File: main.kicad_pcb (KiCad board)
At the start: 2 copper layers, 120 x 100 mm, 21 parts, among them J1 Conn_01x01_Female, J2 Conn_01x01_Female, J3 Conn_01x01_Female, J4 Conn_01x01_Female, J5 Conn_01x01_Female, J6 Conn_01x01_Female, J7 Conn_Coaxial, Q1 AOT2618

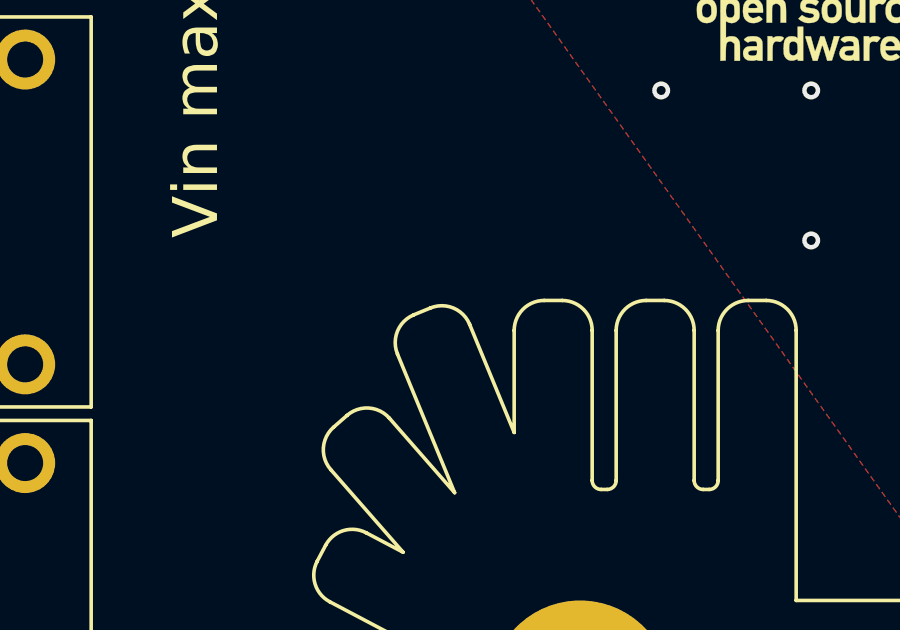
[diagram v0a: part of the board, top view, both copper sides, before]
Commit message: Added BOM
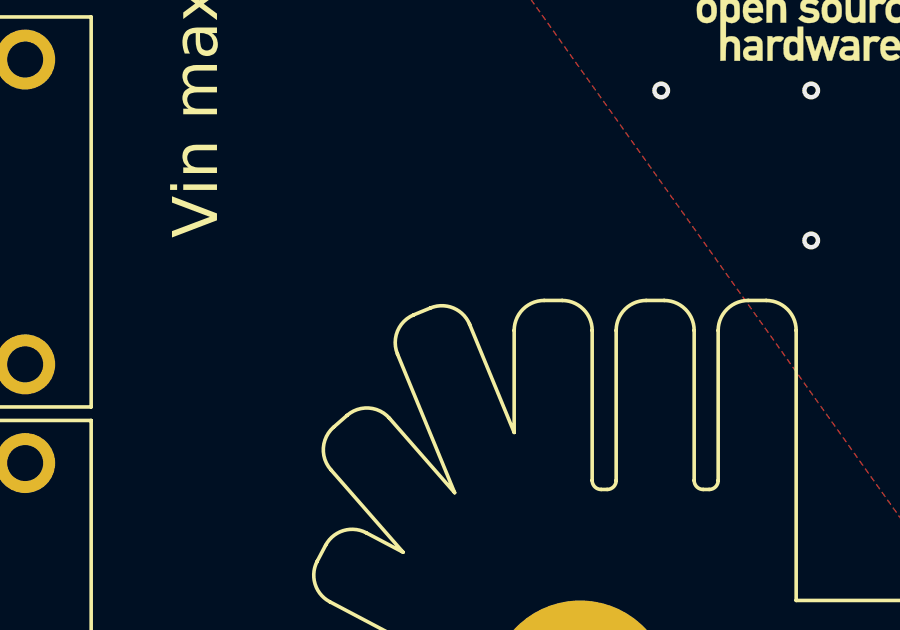
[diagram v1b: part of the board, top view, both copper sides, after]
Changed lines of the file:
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@@
     (descr "CP, Radial series, Radial, pin pitch=5.00mm, , diameter=10mm, Electrolytic Capacitor")
     (tags "CP Radial series Radial pin pitch 5.00mm  diameter 10mm Electrolytic Capacitor")
-    (property "MFN" "Rubycon")
-    (property "PN" "160LEX33MEFC10X16")
+    (property "Alternative" "Rubycon 160LEX33MEFC10X16")
+    (property "MFN" "United Chemicon")
+    (property "PN" "EGXF351ELL330MJ35S")
     (property "Sheetfile" "main.kicad_sch")
     (property "Sheetname" "")
@@
     (descr "Capacitor SMD 1210 (3225 Metric), square (rectangular) end terminal, IPC_7351 nominal, (Body size source: IPC-SM-782 page 76, https://www.pcb-3d.com/wordpress/wp-content/uploads/ipc-sm-782a_amendment_1_and_2.pdf), generated with kicad-footprint-generator")
     (tags "capacitor")
+    (property "Alternative" "TDK CNC6P1X7R2A475K250AE")
     (property "MFN" "TDK")
-    (property "PN" "CNC6P1X7R2A475K250AE")
+    (property "PN" "CNA6P1X7R2A475K250AE")
     (property "Sheetfile" "main.kicad_sch")
     (property "Sheetname" "")
@@
     (descr "CP, Radial series, Radial, pin pitch=7.50mm, , diameter=18mm, Electrolytic Capacitor")
     (tags "CP Radial series Radial pin pitch 7.50mm  diameter 18mm Electrolytic Capacitor")
+    (property "Alternative" "United Chemicon EKYB101ELL102MM40S")
     (property "MFN" "Nichicon")
     (property "PN" "UPW2A102MHD")
@@
     (property "Sheetfile" "main.kicad_sch")
     (property "Sheetname" "")
-    (attr exclude_from_pos_files)
+    (property "exclude_from_bom" "")
+    (attr exclude_from_pos_files exclude_from_bom)
     (fp_text reference "LOGO2" (at 0 0) (layer "F.SilkS") hide
       (effects (font (size 1 1) (thickness 0.15)))
@@
     (descr "Resistor SMD 0805 (2012 Metric), square (rectangular) end terminal, IPC_7351 nominal, (Body size source: IPC-SM-782 page 72, https://www.pcb-3d.com/wordpress/wp-content/uploads/ipc-sm-782a_amendment_1_and_2.pdf), generated with kicad-footprint-generator")
     (tags "resistor")
+    (property "Alternative" "Panasonic ERJ-6ENF1002V")
+    (property "MFN" "Yageo")
+    (property "PN" "AC0805FR-0710KL")
     (property "Sheetfile" "main.kicad_sch")
     (property "Sheetname" "")
@@
     (descr "Capacitor SMD 1206 (3216 Metric), square (rectangular) end terminal, IPC_7351 nominal, (Body size source: IPC-SM-782 page 76, https://www.pcb-3d.com/wordpress/wp-content/uploads/ipc-sm-782a_amendment_1_and_2.pdf), generated with kicad-footprint-generator")
     (tags "capacitor")
+    (property "Alternative" "TDK CGA5L2X7R2A105K160AA")
     (property "MFN" "TDK")
     (property "PN" "CGA5L2X7R2A105M160AE")
@@
     (descr "Capacitor SMD 1206 (3216 Metric), square (rectangular) end terminal, IPC_7351 nominal, (Body size source: IPC-SM-782 page 76, https://www.pcb-3d.com/wordpress/wp-content/uploads/ipc-sm-782a_amendment_1_and_2.pdf), generated with kicad-footprint-generator")
     (tags "capacitor")
+    (property "Alternative" "TDK CGA5L2X7R2A105K160AA")
     (property "MFN" "TDK")
     (property "PN" "CGA5L2X7R2A105M160AE")
@@
     (property "Sheetfile" "main.kicad_sch")
     (property "Sheetname" "")
-    (attr exclude_from_pos_files)
+    (property "exclude_from_bom" "")
+    (attr exclude_from_pos_files exclude_from_bom)
     (fp_text reference "LOGO1" (at 0 0) (layer "F.SilkS") hide
       (effects (font (size 1 1) (thickness 0.15)))
@@
     (fp_arc (start 21.465279 -4.307629) (mid 21.535978 -3.545533) (end 21.047085 -2.956661) (layer "F.SilkS") (width 0.12))
     (fp_arc (start -21.067316 4.100505) (mid -21.145601 3.365146) (end -20.696747 2.777429) (layer "F.SilkS") (width 0.12))
-    (fp_arc (start 19.058317 -9.075185) (mid 19.74445 -9.414242) (end 20.469421 -9.168911) (layer "F.SilkS") (width 0.12))
+    (fp_arc (start 19.058317 -9.075185) (mid 19.74446 -9.41424) (end 20.469421 -9.168911) (layer "F.SilkS") (width 0.12))
     (fp_arc (start 16.386175 -12.20573) (mid 16.926425 -12.747869) (end 17.691791 -12.749206) (layer "F.SilkS") (width 0.12))
     (fp_arc (start -8.1 -7) (mid -8.187868 -6.787868) (end -8.4 -6.7) (layer "F.SilkS") (width 0.12))
@@
     (fp_arc (start 10.5 -13) (mid 11.207107 -12.707107) (end 11.5 -12) (layer "F.SilkS") (width 0.12))
     (fp_arc (start 14.8 11.9) (mid 14.507107 12.607107) (end 13.8 12.9) (layer "F.SilkS") (width 0.12))
-    (fp_arc (start -17.691791 -12.749206) (mid -16.926426 -12.74787) (end -16.386175 -12.20573) (layer "F.SilkS") (width 0.12))
+    (fp_arc (start -17.691791 -12.749206) (mid -16.926425 -12.74787) (end -16.386175 -12.20573) (layer "F.SilkS") (width 0.12))
     (fp_arc (start 20.774322 9.592377) (mid 20.052858 9.847847) (end 19.362046 9.518363) (layer "F.SilkS") (width 0.12))
     (fp_arc (start -21.047085 -2.956661) (mid -21.535977 -3.545534) (end -21.465279 -4.307629) (layer "F.SilkS") (width 0.12))
@@
     (fp_arc (start 8.4 -6.2) (mid 7.834315 -6.434315) (end 7.6 -7) (layer "F.Fab") (width 0.1))
     (fp_arc (start -11 -11.8) (mid -10.803962 -12.285821) (end -10.325651 -12.49953) (layer "F.Fab") (width 0.1))
-    (fp_arc (start 12.79953 -11.8) (mid 13.004551 -12.294999) (end 13.49953 -12.5) (layer "F.Fab") (width 0.1))
+    (fp_arc (start 12.79953 -11.8) (mid 13.004541 -12.294989) (end 13.49953 -12.5) (layer "F.Fab") (width 0.1))
     (fp_arc (start 12.8 -7) (mid 12.565685 -6.434315) (end 12 -6.2) (layer "F.Fab") (width 0.1))
     (fp_arc (start 13.374349 12.49953) (mid 12.896038 12.285821) (end 12.7 11.8) (layer "F.Fab") (width 0.1))
     (fp_arc (start 11.8 -6.2) (mid 11.234315 -6.434315) (end 11 -7) (layer "F.Fab") (width 0.1))
     (fp_arc (start -12 -6.2) (mid -12.565685 -6.434315) (end -12.8 -7) (layer "F.Fab") (width 0.1))
-    (fp_arc (start 13.725181 -12.49953) (mid 14.203509 -12.285818) (end 14.39953 -11.8) (layer "F.Fab") (width 0.1))
+    (fp_arc (start 13.725181 -12.49953) (mid 14.203536 -12.285845) (end 14.39953 -11.8) (layer "F.Fab") (width 0.1))
     (fp_arc (start -13.49953 -12.5) (mid -13.004555 -12.294975) (end -12.79953 -11.8) (layer "F.Fab") (width 0.1))
     (fp_arc (start -14.39953 -11.8) (mid -14.203492 -12.285821) (end -13.725181 -12.49953) (layer "F.Fab") (width 0.1))
     (fp_arc (start -13.60047 12.5) (mid -14.095445 12.294975) (end -14.30047 11.8) (layer "F.Fab") (width 0.1))
-    (fp_arc (start 14.30047 11.8) (mid 14.095449 12.294999) (end 13.60047 12.5) (layer "F.Fab") (width 0.1))
+    (fp_arc (start 14.30047 11.8) (mid 14.095459 12.294989) (end 13.60047 12.5) (layer "F.Fab") (width 0.1))
     (fp_arc (start -7.6 -7) (mid -7.834315 -6.434315) (end -8.4 -6.2) (layer "F.Fab") (width 0.1))
     (fp_arc (start 6.925651 -12.49953) (mid 7.403962 -12.285821) (end 7.6 -11.8) (layer "F.Fab") (width 0.1))
@@
     (descr "Resistor SMD 1206 (3216 Metric), square (rectangular) end terminal, IPC_7351 nominal, (Body size source: IPC-SM-782 page 72, https://www.pcb-3d.com/wordpress/wp-content/uploads/ipc-sm-782a_amendment_1_and_2.pdf), generated with kicad-footprint-generator")
     (tags "resistor")
-    (property "MFN" "Susumu")
-    (property "PN" "RG3216P-49R9-B-T5")
+    (property "Alternative" "Panasonic ERJ-U08F49R9V")
+    (property "MFN" "Yageo")
+    (property "PN" "AC1206FR-0749R9L")
     (property "Sheetfile" "main.kicad_sch")
     (property "Sheetname" "")
@@
     (descr "Resistor SMD 1206 (3216 Metric), square (rectangular) end terminal, IPC_7351 nominal, (Body size source: IPC-SM-782 page 72, https://www.pcb-3d.com/wordpress/wp-content/uploads/ipc-sm-782a_amendment_1_and_2.pdf), generated with kicad-footprint-generator")
     (tags "resistor")
-    (property "MFN" "Susumu")
-    (property "PN" "RG3216P-49R9-B-T5")
+    (property "Alternative" "Panasonic ERJ-U08F49R9V")
+    (property "MFN" "Yageo")
+    (property "PN" "AC1206FR-0749R9L")
     (property "Sheetfile" "main.kicad_sch")
     (property "Sheetname" "")
@@
     (descr "Resistor SMD 1206 (3216 Metric), square (rectangular) end terminal, IPC_7351 nominal, (Body size source: IPC-SM-782 page 72, https://www.pcb-3d.com/wordpress/wp-content/uploads/ipc-sm-782a_amendment_1_and_2.pdf), generated with kicad-footprint-generator")
     (tags "resistor")
-    (property "MFN" "Susumu")
-    (property "PN" "RG3216P-49R9-B-T5")
+    (property "Alternative" "Panasonic ERJ-U08F49R9V")
+    (property "MFN" "Yageo")
+    (property "PN" "AC1206FR-0749R9L")
     (property "Sheetfile" "main.kicad_sch")
     (property "Sheetname" "")
